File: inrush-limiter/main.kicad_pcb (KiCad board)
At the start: 2 copper layers, 30 parts, among them K1 RELAY_2RT, P1 CONN_01X04, Q1 PN2222A, Q2 PN2222A, U1 LM393

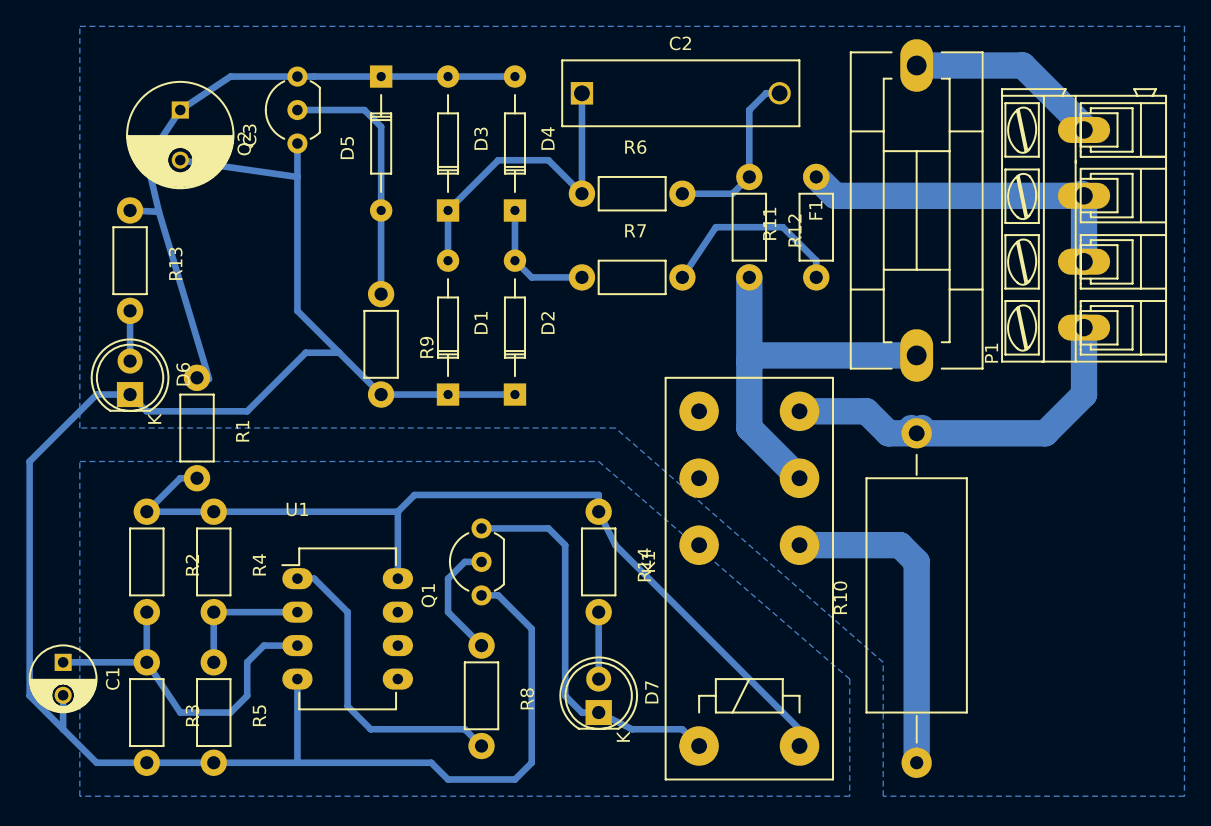
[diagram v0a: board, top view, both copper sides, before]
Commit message: update
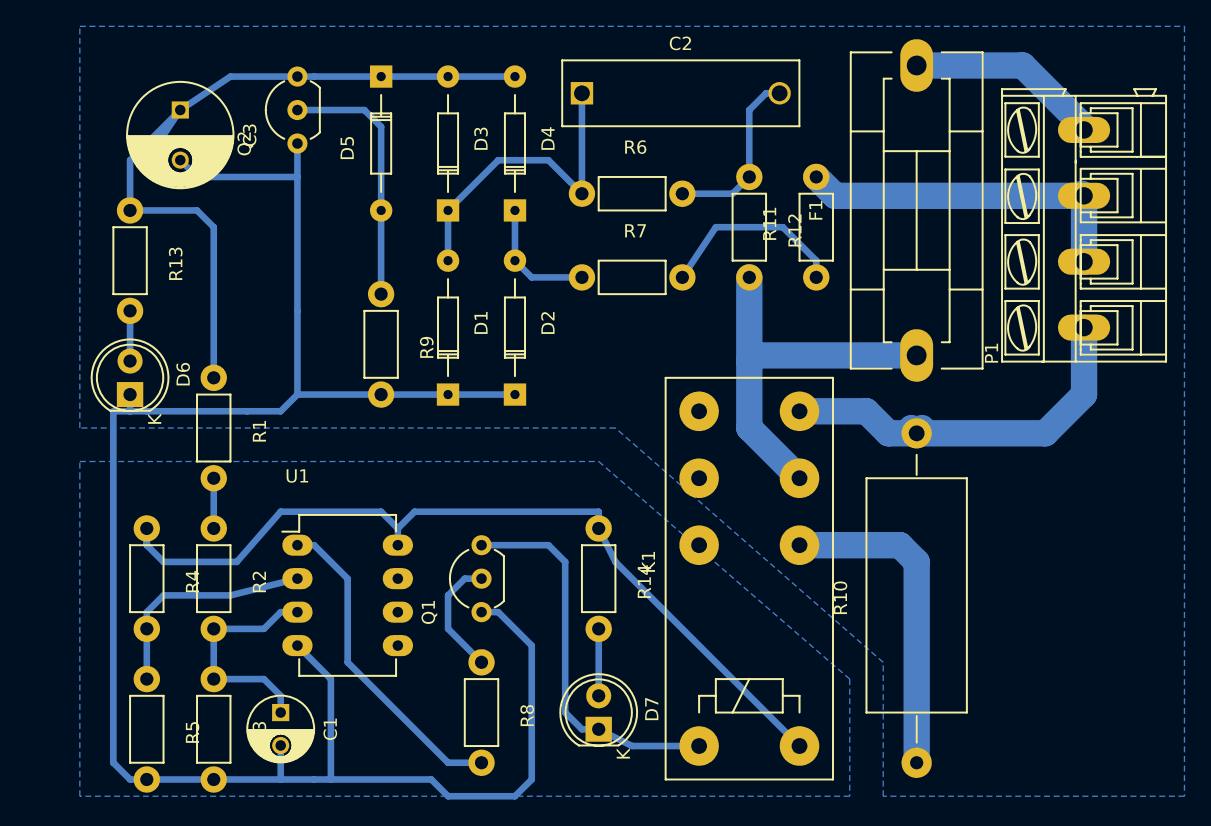
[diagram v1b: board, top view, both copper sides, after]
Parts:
- moved C1 16.9 mm to (129.5, 91.4)
- moved R3 5.24 mm to (124.5, 88.9)
- moved R5 5.24 mm to (119.4, 88.9)
- moved R2 5.24 mm to (124.5, 77.5)
- moved R4 5.24 mm to (119.4, 77.5)
- moved U1 2.54 mm to (130.8, 78.7)
- moved D7 1.27 mm to (153.7, 92.7)
- moved Q1 1.27 mm to (144.8, 83.8)
- moved R1 1.27 mm to (124.5, 66.0)
- moved R14 1.27 mm to (153.7, 77.5)
- moved R8 1.27 mm to (144.8, 87.6)
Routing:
- net Net-(C1-Pad1): track 27.2 -> 17.6 mm
- net +5V: track 50.2 -> 58.3 mm
- net Net-(R4-Pad2): track 10.2 -> 17.2 mm
- net Net-(K1-PadA2): track 60.0 -> 66.5 mm
- net Net-(R1-Pad2): track 9.94 -> 3.81 mm
- net GND: track 151.9 -> 149.7 mm
- net Net-(D7-Pad1): track 31.1 -> 29.3 mm
- net Net-(R8-Pad2): track 23.4 -> 24.5 mm
